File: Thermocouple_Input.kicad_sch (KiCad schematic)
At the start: 7 parts, among them J1 12-24V POWER IN, U1 N7805-1PH, U2 N7803-1PH

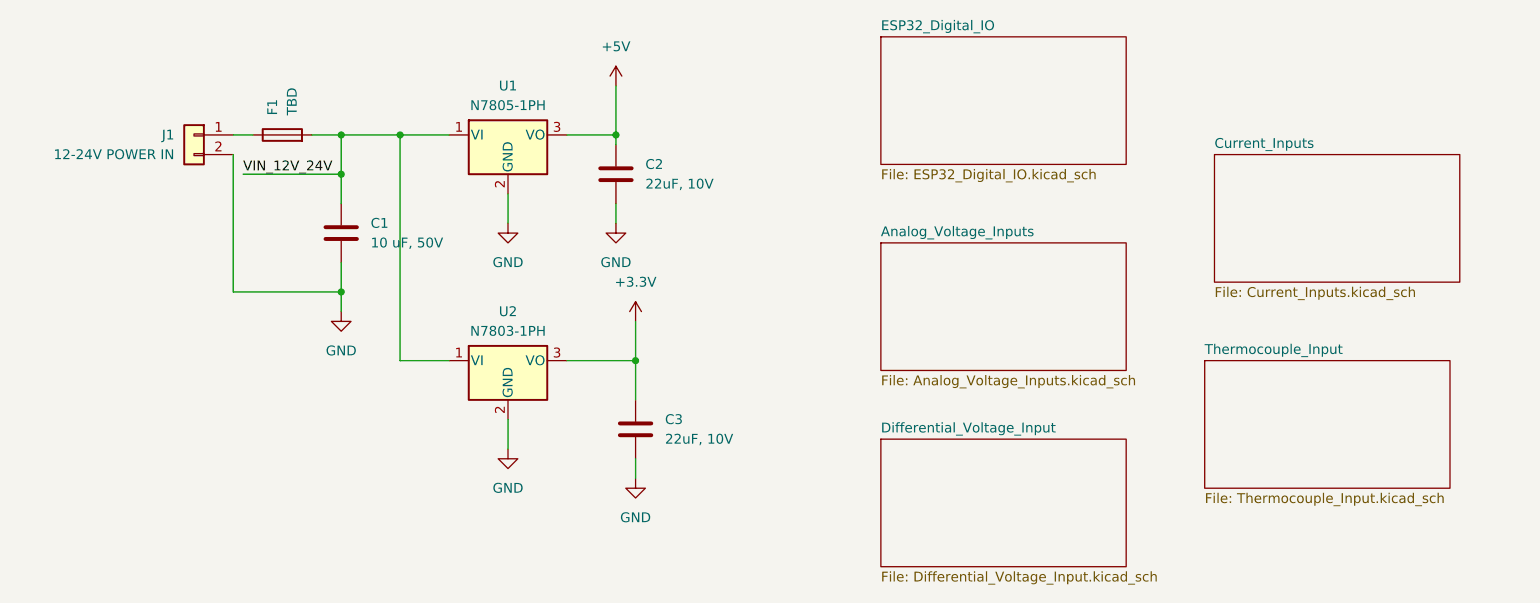
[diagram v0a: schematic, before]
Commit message: added remaining pages. BOM and refinement is all thats left
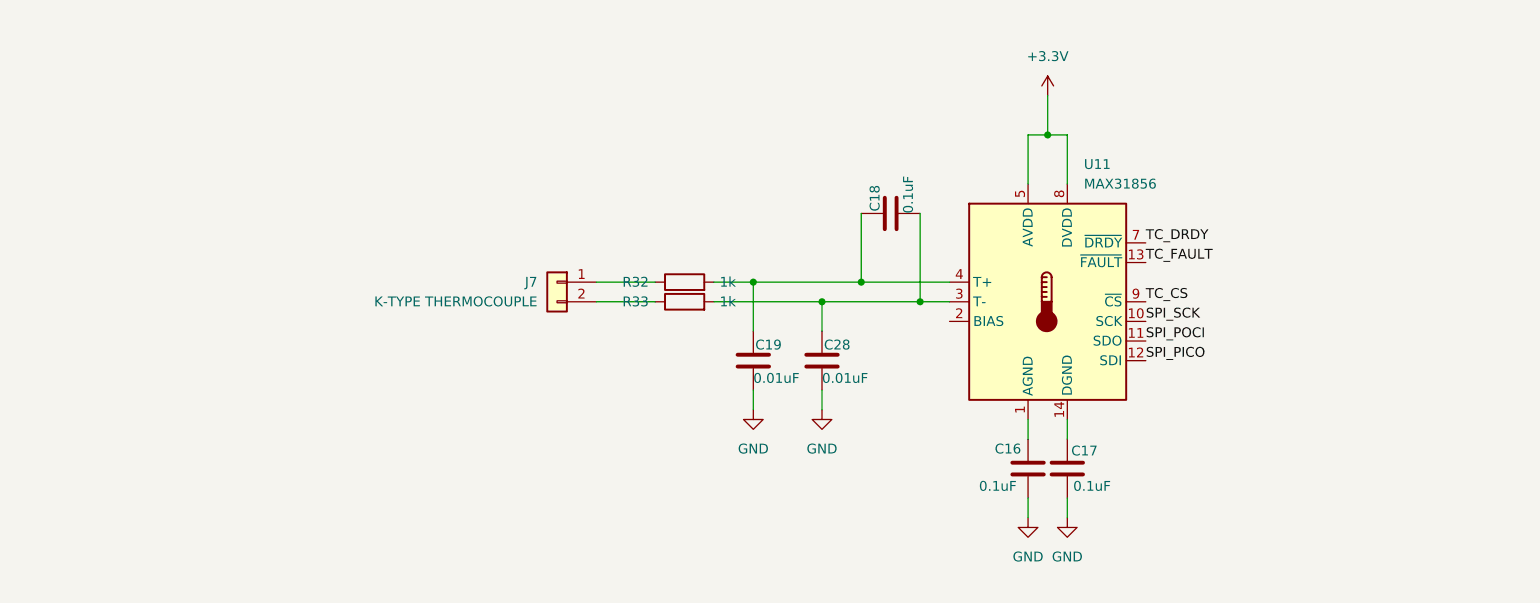
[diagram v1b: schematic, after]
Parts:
- removed C1: 10 uF, 50V, symbol Device:C
- removed C2, C3: 22uF, 10V, symbol Device:C
- removed F1: TBD, symbol Device:Fuse
- removed J1: 12-24V POWER IN, symbol Connector_Generic:Conn_01x02
- removed U1: N7805-1PH, Package_TO_SOT_THT:TO-220-3_Vertical, symbol Regulator_Linear:LM7805_TO220
- removed U2: N7803-1PH, Package_TO_SOT_THT:TO-220-3_Vertical, symbol Regulator_Linear:LM7805_TO220
- added C16, C17, C18: 0.1uF, Package_SO:TSSOP-14_4.4x5mm_P0.65mm, symbol Device:C
- added C19, C28: 0.01uF, Package_SO:TSSOP-14_4.4x5mm_P0.65mm, symbol Device:C
- added J7: K-TYPE THERMOCOUPLE, symbol Connector_Generic:Conn_01x02
- added R32, R33: 1k, symbol Device:R
- added U11: MAX31856, Package_SO:TSSOP-14_4.4x5mm_P0.65mm, symbol Sensor_Temperature:MAX31856
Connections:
- net +3.3V: now also U11.5 (AVDD), U11.8 (DVDD)
- net GND: now also C16.2, C17.2, C19.2, C28.2
- new net: C18.1, C19.1, R32.2, U11.4 (T+)
- new net: C18.2, C28.1, R33.2, U11.3 (T-)
- new net: C16.1, U11.1 (AGND)
- new net: C17.1, U11.14 (DGND)
- new net: J7.1 (Pin_1), R32.1
- new net: J7.2 (Pin_2), R33.1
- new net SPI_PICO: U11.12 (SDI)
- new net SPI_POCI: U11.11 (SDO)
- new net SPI_SCK: U11.10 (SCK)
- new net TC_CS: U11.9 (~{CS})
- new net TC_DRDY: U11.7 (~{DRDY})
- new net TC_FAULT: U11.13 (~{FAULT})
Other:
- removed sheet Analog_Voltage_Inputs
- removed sheet Current_Inputs
- removed sheet Differential_Voltage_Input
- removed sheet ESP32_Digital_IO
- removed sheet Thermocouple_Input
- company: Faster Than Sound -> Slap DAQ
- title: System/Power -> Thermocouple Input
